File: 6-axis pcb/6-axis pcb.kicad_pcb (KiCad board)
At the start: 2 copper layers, 80 x 140 mm, 28 parts, among them J1 Conn_01x04_Pin, J2 Conn_01x04_Pin, J3 Conn_01x04_Pin, J4 Conn_01x04_Pin, J5 Conn_01x04_Pin, J6 Conn_01x04_Pin, U1 ESP32-C6-DEVKITC-1-N8

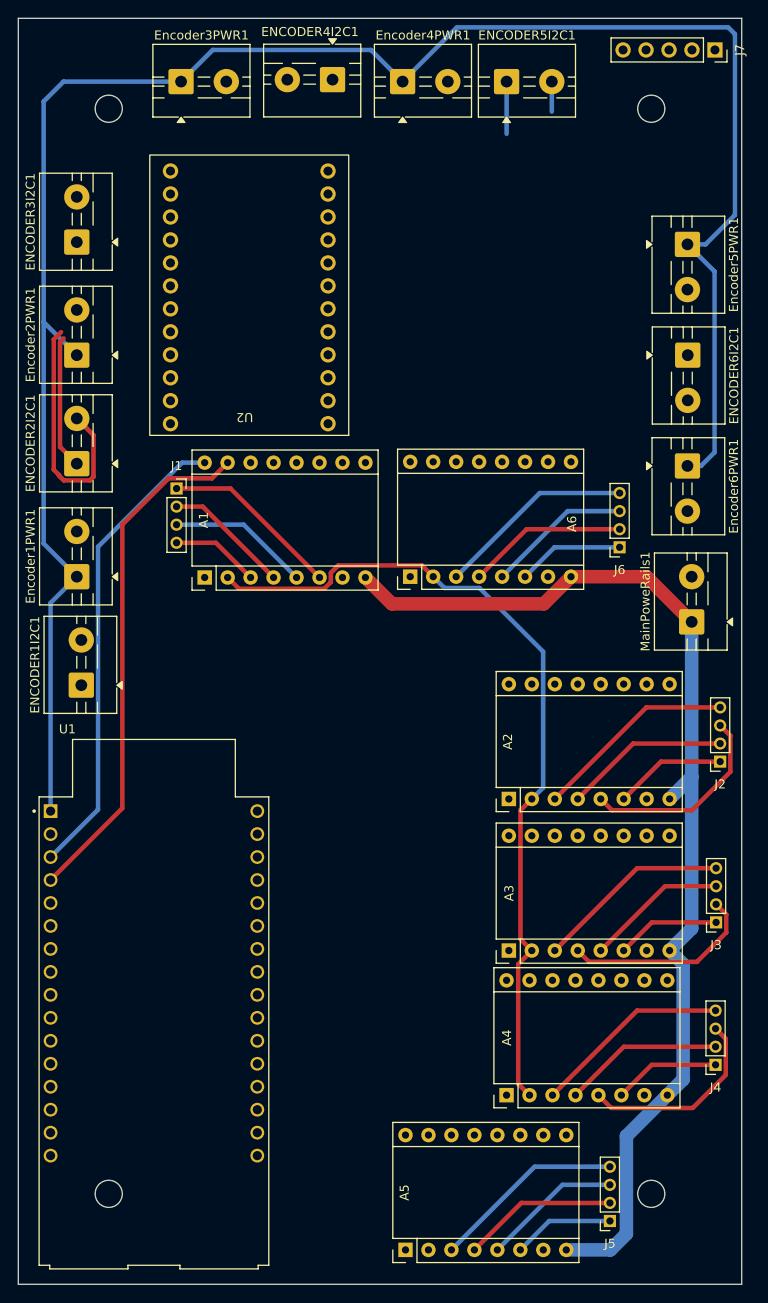
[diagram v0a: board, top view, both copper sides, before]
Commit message: Move to Laptop
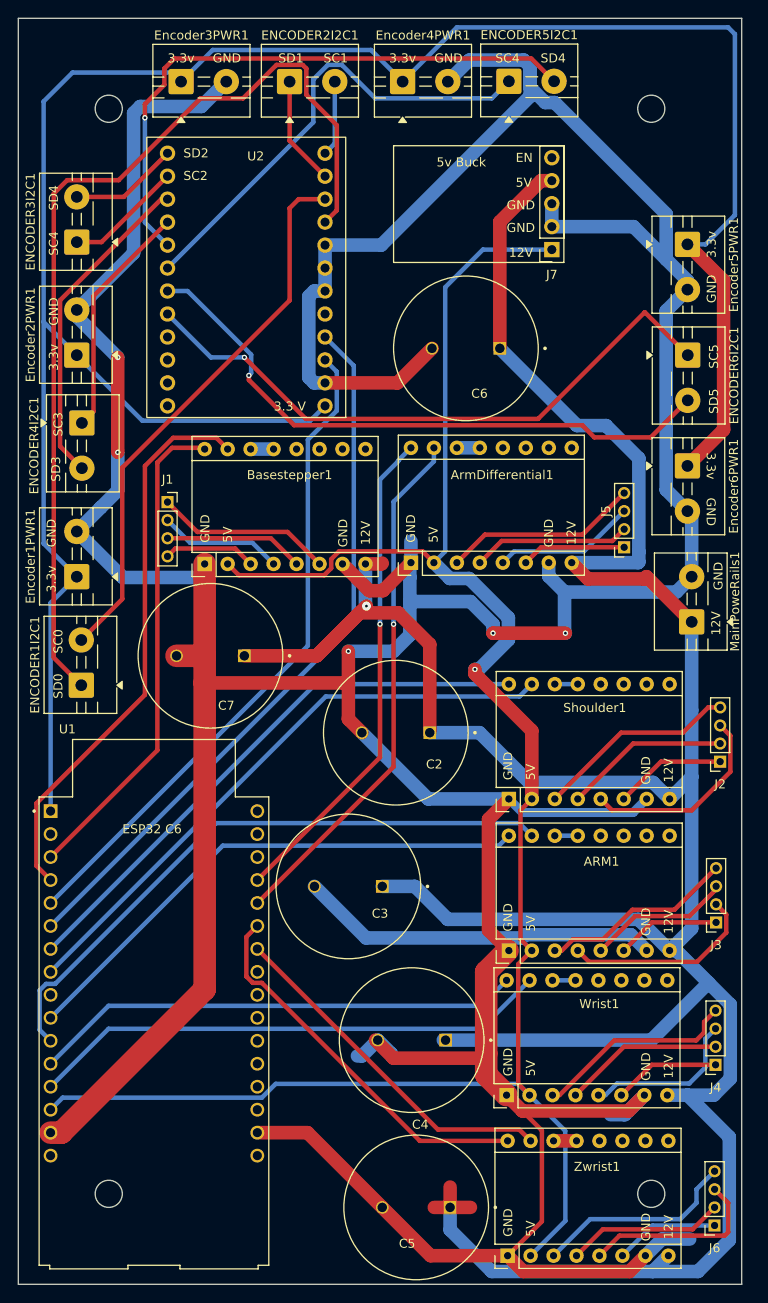
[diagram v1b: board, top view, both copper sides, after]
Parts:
- added C2: EEUFK1V102S, 5x12 electrolytic capacitor:CAPPRD750W80D1600H1500, F.Cu at (66.8, 109.0)
- added C3: EEUFK1V102S, 5x12 electrolytic capacitor:CAPPRD750W80D1600H1500, F.Cu at (61.5, 126.0)
- added C4: EEUFK1V102S, 5x12 electrolytic capacitor:CAPPRD750W80D1600H1500, F.Cu at (68.5, 143.0)
- added C5: EEUFK1V102S, 5x12 electrolytic capacitor:CAPPRD750W80D1600H1500, F.Cu at (69.0, 161.5)
- added C6: EEUFK1V102S, 5x12 electrolytic capacitor:CAPPRD750W80D1600H1500, F.Cu at (74.5, 66.5)
- added C7: EEUFK1V102S, 5x12 electrolytic capacitor:CAPPRD750W80D1600H1500, F.Cu at (46.2, 100.5)
- moved ArmDifferential1 76.0 mm to (68.4, 90.2)
- moved Zwrist1 75.9 mm to (79.1, 166.8)
- moved J6 75.7 mm to (102.0, 163.5)
- moved J5 74.5 mm to (92.0, 88.5)
- moved ENCODER2I2C1 48.4 mm to (55.0, 37.0), turned to 0 degrees
- moved ENCODER4I2C1 47.0 mm to (32.0, 74.8), turned to -90 degrees
- moved J7 28.5 mm to (84.0, 55.6), turned to 180 degrees
- moved U2 2.00 mm to (61.2, 74.2)
- moved J1 1.80 mm to (41.5, 83.5)
- moved Basestepper1 1.50 mm to (45.6, 90.3)
- moved ENCODER5I2C1 0.25 mm to (79.2, 37.0)
- renumbered A3 to ARM1, A5 to ArmDifferential1, A1 to Basestepper1, A2 to Shoulder1, A4 to Wrist1, A6 to Zwrist1
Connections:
- ARM1 pad 13: unconnected-(A3-~{RESET}-Pad13) -> Net-(ARM1-~{RESET})
- ARM1 pad 14: Net-(A3-~{ENABLE}) -> Net-(ARM1-~{RESET})
- ARM1 pad 9: Net-(A3-~{ENABLE}) -> unconnected-(ARM1-~{ENABLE}-Pad9)
- ArmDifferential1 pad 13: unconnected-(A5-~{RESET}-Pad13) -> Net-(ArmDifferential1-~{RESET})
- ArmDifferential1 pad 14: Net-(A5-~{ENABLE}) -> Net-(ArmDifferential1-~{RESET})
- ArmDifferential1 pad 9: Net-(A5-~{ENABLE}) -> unconnected-(ArmDifferential1-~{ENABLE}-Pad9)
- Basestepper1 pad 13: unconnected-(A1-~{RESET}-Pad13) -> Net-(Basestepper1-~{RESET})
- Basestepper1 pad 14: Net-(A1-~{ENABLE}) -> Net-(Basestepper1-~{RESET})
- Basestepper1 pad 9: Net-(A1-~{ENABLE}) -> unconnected-(Basestepper1-~{ENABLE}-Pad9)
- J7 pad 1: +12V -> +5V
- J7 pad 4: +5V -> +12V
- Shoulder1 pad 13: unconnected-(A2-~{RESET}-Pad13) -> Net-(Shoulder1-~{RESET})
- Shoulder1 pad 14: Net-(A2-~{ENABLE}) -> Net-(Shoulder1-~{RESET})
- Shoulder1 pad 9: Net-(A2-~{ENABLE}) -> unconnected-(Shoulder1-~{ENABLE}-Pad9)
- Wrist1 pad 13: unconnected-(A4-~{RESET}-Pad13) -> Net-(Wrist1-~{RESET})
- Wrist1 pad 14: Net-(A4-~{ENABLE}) -> Net-(Wrist1-~{RESET})
- Wrist1 pad 9: Net-(A4-~{ENABLE}) -> unconnected-(Wrist1-~{ENABLE}-Pad9)
- Zwrist1 pad 13: unconnected-(A6-~{RESET}-Pad13) -> Net-(Zwrist1-~{RESET})
- Zwrist1 pad 14: Net-(A6-~{ENABLE}) -> Net-(Zwrist1-~{RESET})
- Zwrist1 pad 9: Net-(A6-~{ENABLE}) -> unconnected-(Zwrist1-~{ENABLE}-Pad9)
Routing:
- net GND: track 0.00 -> 636.1 mm, vias 0 -> 5
- net +12V: track 123.3 -> 350.6 mm, vias 0 -> 1
- net +5V: track 92.8 -> 215.8 mm, vias 0 -> 1
- net /SD0: track 0.00 -> 108.5 mm
- net /SCL: track 0.00 -> 80.3 mm
- net /SDA: track 0.00 -> 73.7 mm
- net /SC5: track 0.00 -> 69.2 mm, vias 0 -> 1
- net /GPIO11: track 0.00 -> 68.7 mm
- net /SD5: track 0.00 -> 67.9 mm, vias 0 -> 1
- net /GPIO1: track 0.00 -> 66.4 mm
- net /GPIO0: track 0.00 -> 62.8 mm
- net /<NO NET>: track 3.32 -> 66.1 mm, vias 0 -> 1
- net /SC0: track 0.00 -> 61.6 mm
- net /GPIO10: track 0.00 -> 59.0 mm
- net /GPIO23: track 0.00 -> 58.4 mm, vias 0 -> 1
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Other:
- board text added: "12V"
- board text added: "3.3 V"
- board text added: "3.3v"
- board text added: "5V"
- board text added: "5v Buck"
- board text added: "EN"
- board text added: "ESP32 C6"
- board text added: "GND"
- board text added: "SC0"
- board text added: "SC1"
- board text added: "SC2"
- board text added: "SC3"
- board text added: "SC4"
- board text added: "SC5"
- board text added: "SD0"
- board text added: "SD1"
- board text added: "SD2"
- board text added: "SD3"
- board text added: "SD4"
- board text added: "SD5"
